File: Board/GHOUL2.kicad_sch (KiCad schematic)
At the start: 32 parts, among them M1 Motor_Servo, U1 Teensy4.1, U2 DS18S20, U4 TPS62133, U5 MS5607-02BA, U6 SAM-M8Q

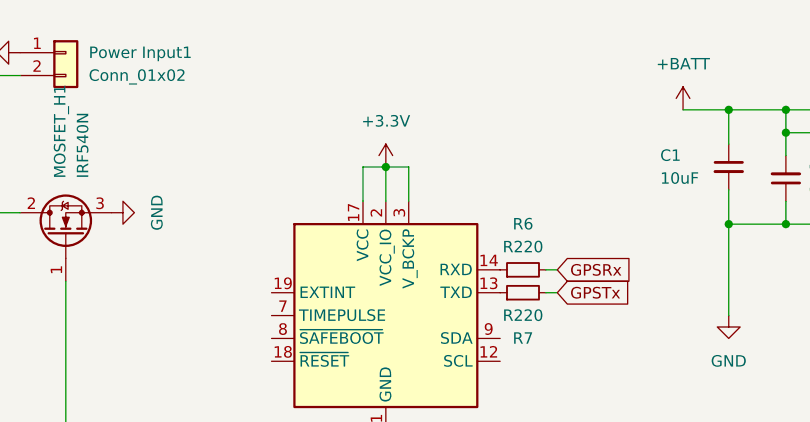
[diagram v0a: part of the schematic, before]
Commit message: decoupling and gps batt
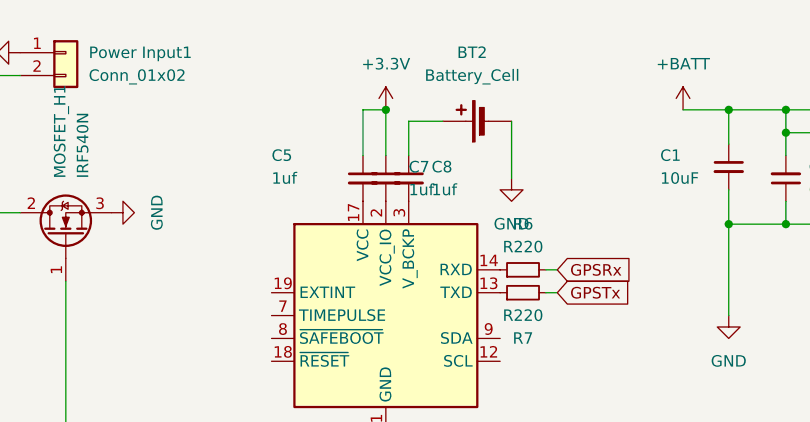
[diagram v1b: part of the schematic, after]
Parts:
- added BT2: Battery_Cell, Battery:BatteryHolder_Keystone_2998_1x6.8mm, symbol Device:Battery_Cell
- added C5, C7, C8: 1uf, Capacitor_SMD:C_0201_0603Metric_Pad0.64x0.40mm_HandSolder, symbol Device:C_Small
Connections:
- net +3.3V: now also C5.1, C7.1; no longer U6.17 (VCC), U6.2 (VCC_IO), U6.3 (V_BCKP)
- net GND: now also BT2.2 (-)
- new net: C5.2, U6.17 (VCC)
- new net: BT2.1 (+), C8.1
- new net: C7.2, U6.2 (VCC_IO)
- new net: C8.2, U6.3 (V_BCKP)
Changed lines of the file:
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@@
   (junction (at 240.03 54.61) (diameter 0) (color 0 0 0 0)
   )
-  (junction (at 166.37 31.75) (diameter 0) (color 0 0 0 0)
-  )
   (junction (at 256.54 43.18) (diameter 0) (color 0 0 0 0)
   )
@@
   (junction (at 30.48 148.59) (diameter 0) (color 0 0 0 0)
   )
+  (junction (at 166.37 25.4) (diameter 0) (color 0 0 0 0)
+  )
   (junction (at 107.95 143.51) (diameter 0) (color 0 0 0 0)
   )
@@
     (stroke (width 0) (type default))
   )
+  (wire (pts (xy 172.72 26.67) (xy 168.91 26.67))
+    (stroke (width 0) (type default))
+  )
   (wire (pts (xy 240.03 54.61) (xy 237.49 54.61))
     (stroke (width 0) (type default))
@@
     (stroke (width 0) (type default))
   )
+  (wire (pts (xy 180.34 26.67) (xy 180.34 33.02))
+    (stroke (width 0) (type default))
+  )
   (wire (pts (xy 30.48 148.59) (xy 53.34 148.59))
     (stroke (width 0) (type default))
@@
     (stroke (width 0) (type default))
   )
+  (wire (pts (xy 163.83 30.48) (xy 163.83 25.4))
+    (stroke (width 0) (type default))
+  )
   (wire (pts (xy 237.49 53.34) (xy 237.49 54.61))
     (stroke (width 0) (type default))
@@
     (stroke (width 0) (type default))
   )
-  (wire (pts (xy 163.83 35.56) (xy 163.83 31.75))
-    (stroke (width 0) (type default))
-  )
   (wire (pts (xy 26.67 168.91) (xy 29.21 168.91))
     (stroke (width 0) (type default))
@@
     (stroke (width 0) (type default))
   )
-  (wire (pts (xy 166.37 31.75) (xy 168.91 31.75))
-    (stroke (width 0) (type default))
-  )
   (wire (pts (xy 26.67 148.59) (xy 26.67 156.21))
     (stroke (width 0) (type default))
@@
     (stroke (width 0) (type default))
   )
-  (wire (pts (xy 168.91 31.75) (xy 168.91 35.56))
-    (stroke (width 0) (type default))
-  )
   (wire (pts (xy 218.44 142.24) (xy 219.71 142.24))
     (stroke (width 0) (type default))
@@
     (stroke (width 0) (type default))
   )
-  (wire (pts (xy 163.83 31.75) (xy 166.37 31.75))
-    (stroke (width 0) (type default))
-  )
   (wire (pts (xy 115.57 21.59) (xy 125.73 21.59))
     (stroke (width 0) (type default))
@@
     (stroke (width 0) (type default))
   )
+  (wire (pts (xy 168.91 26.67) (xy 168.91 30.48))
+    (stroke (width 0) (type default))
+  )
   (wire (pts (xy 222.25 43.18) (xy 227.33 43.18))
     (stroke (width 0) (type default))
@@
     (stroke (width 0) (type default))
   )
-  (wire (pts (xy 166.37 31.75) (xy 166.37 35.56))
+  (wire (pts (xy 166.37 25.4) (xy 166.37 30.48))
     (stroke (width 0) (type default))
   )
@@
   )
   (wire (pts (xy 237.49 54.61) (xy 234.95 54.61))
+    (stroke (width 0) (type default))
+  )
+  (wire (pts (xy 163.83 25.4) (xy 166.37 25.4))
     (stroke (width 0) (type default))
   )
@@
     (property "Intersheetrefs" "${INTERSHEET_REFS}" (at 27.495 41.91 0)
       (effects (font (size 1.27 1.27)) (justify right) hide)
+    )
+  )
+  (symbol (lib_id "Device:C_Small") (at 163.83 33.02 0) (unit 1)
+    (in_bom yes) (on_board yes) (dnp no)
+    (property "Reference" "C5" (at 153.67 30.48 0)
+      (effects (font (size 1.27 1.27)) (justify left))
+    )
+    (property "Value" "1uf" (at 153.67 33.02 0)
+      (effects (font (size 1.27 1.27)) (justify left))
+    )
+    (property "Footprint" "Capacitor_SMD:C_0201_0603Metric_Pad0.64x0.40mm_HandSolder" (at 163.83 33.02 0)
+      (effects (font (size 1.27 1.27)) hide)
+    )
+    (property "Datasheet" "~" (at 163.83 33.02 0)
+      (effects (font (size 1.27 1.27)) hide)
+    )
+    (pin "1")
+    (pin "2")
+    (instances
+      (project "GHOUL2"
+        (path "/a2e390a1-3d20-4e85-b6dd-da84eefdc6ca"
+          (reference "C5") (unit 1)
+        )
+      )
     )
   )
@@
         (path "/a2e390a1-3d20-4e85-b6dd-da84eefdc6ca"
           (reference "#PWR07") (unit 1)
+        )
+      )
+    )
+  )
+  (symbol (lib_id "Device:Battery_Cell") (at 177.8 26.67 90) (unit 1)
+    (in_bom yes) (on_board yes) (dnp no) (fields_autoplaced)
+    (property "Reference" "BT2" (at 175.9585 19.05 90)
+      (effects (font (size 1.27 1.27)))
+    )
+    (property "Value" "Battery_Cell" (at 175.9585 21.59 90)
+      (effects (font (size 1.27 1.27)))
+    )
+    (property "Footprint" "Battery:BatteryHolder_Keystone_2998_1x6.8mm" (at 176.276 26.67 90)
+      (effects (font (size 1.27 1.27)) hide)
+    )
+    (property "Datasheet" "~" (at 176.276 26.67 90)
+      (effects (font (size 1.27 1.27)) hide)
+    )
+    (pin "1")
+    (pin "2")
+    (instances
+      (project "GHOUL2"
+        (path "/a2e390a1-3d20-4e85-b6dd-da84eefdc6ca"
+          (reference "BT2") (unit 1)
         )
       )
@@
     )
   )
+  (symbol (lib_id "Device:C_Small") (at 166.37 33.02 0) (unit 1)
+    (in_bom yes) (on_board yes) (dnp no) (fields_autoplaced)
+    (property "Reference" "C7" (at 168.91 31.7563 0)
+      (effects (font (size 1.27 1.27)) (justify left))
+    )
+    (property "Value" "1uf" (at 168.91 34.2963 0)
+      (effects (font (size 1.27 1.27)) (justify left))
+    )
+    (property "Footprint" "Capacitor_SMD:C_0201_0603Metric_Pad0.64x0.40mm_HandSolder" (at 166.37 33.02 0)
+      (effects (font (size 1.27 1.27)) hide)
+    )
+    (property "Datasheet" "~" (at 166.37 33.02 0)
+      (effects (font (size 1.27 1.27)) hide)
+    )
+    (pin "1")
+    (pin "2")
+    (instances
+      (project "GHOUL2"
+        (path "/a2e390a1-3d20-4e85-b6dd-da84eefdc6ca"
+          (reference "C7") (unit 1)
+        )
+      )
+    )
+  )
   (symbol (lib_id "power:GND") (at 143.51 120.65 270) (unit 1)
     (in_bom yes) (on_board yes) (dnp no)
@@
     )
   )
+  (symbol (lib_name "GND_8") (lib_id "power:GND") (at 180.34 33.02 0) (unit 1)
+    (in_bom yes) (on_board yes) (dnp no) (fields_autoplaced)
+    (property "Reference" "#PWR023" (at 180.34 39.37 0)
+      (effects (font (size 1.27 1.27)) hide)
+    )
+    (property "Value" "GND" (at 180.34 38.1 0)
+      (effects (font (size 1.27 1.27)))
+    )
+    (property "Footprint" "" (at 180.34 33.02 0)
+      (effects (font (size 1.27 1.27)) hide)
+    )
+    (property "Datasheet" "" (at 180.34 33.02 0)
+      (effects (font (size 1.27 1.27)) hide)
+    )
+    (pin "1")
+    (instances
+      (project "GHOUL2"
+        (path "/a2e390a1-3d20-4e85-b6dd-da84eefdc6ca"
+          (reference "#PWR023") (unit 1)
+        )
+      )
+    )
+  )
   (symbol (lib_id "power:GND") (at 156.21 88.9 90) (unit 1)
     (in_bom yes) (on_board yes) (dnp no)
@@
     )
   )
-  (symbol (lib_id "power:+3.3V") (at 166.37 31.75 0) (unit 1)
-    (in_bom yes) (on_board yes) (dnp no) (fields_autoplaced)
-    (property "Reference" "#PWR014" (at 166.37 35.56 0)
-      (effects (font (size 1.27 1.27)) hide)
-    )
-    (property "Value" "+3.3V" (at 166.37 26.67 0)
-      (effects (font (size 1.27 1.27)))
-    )
-    (property "Footprint" "" (at 166.37 31.75 0)
-      (effects (font (size 1.27 1.27)) hide)
-    )
-    (property "Datasheet" "" (at 166.37 31.75 0)
+  (symbol (lib_id "power:+3.3V") (at 166.37 25.4 0) (unit 1)
+    (in_bom yes) (on_board yes) (dnp no) (fields_autoplaced)
+    (property "Reference" "#PWR014" (at 166.37 29.21 0)
+      (effects (font (size 1.27 1.27)) hide)
+    )
+    (property "Value" "+3.3V" (at 166.37 20.32 0)
+      (effects (font (size 1.27 1.27)))
+    )
+    (property "Footprint" "" (at 166.37 25.4 0)
+      (effects (font (size 1.27 1.27)) hide)
+    )
+    (property "Datasheet" "" (at 166.37 25.4 0)
       (effects (font (size 1.27 1.27)) hide)
     )
@@
         )
       )
+    )
+  )
+  (symbol (lib_id "Device:C_Small") (at 168.91 33.02 0) (unit 1)
+    (in_bom yes) (on_board yes) (dnp no) (fields_autoplaced)
+    (property "Reference" "C8" (at 171.45 31.7563 0)
+      (effects (font (size 1.27 1.27)) (justify left))
+    )
+    (property "Value" "1uf" (at 171.45 34.2963 0)
+      (effects (font (size 1.27 1.27)) (justify left))
+    )
+    (property "Footprint" "Capacitor_SMD:C_0201_0603Metric_Pad0.64x0.40mm_HandSolder" (at 168.91 33.02 0)
+      (effects (font (size 1.27 1.27)) hide)
+    )
+    (property "Datasheet" "~" (at 168.91 33.02 0)
+      (effects (font (size 1.27 1.27)) hide)
+    )
+    (pin "1")
+    (pin "2")
+    (instances
+      (project "GHOUL2"
+        (path "/a2e390a1-3d20-4e85-b6dd-da84eefdc6ca"
+          (reference "C8") (unit 1)
+        )
+      )

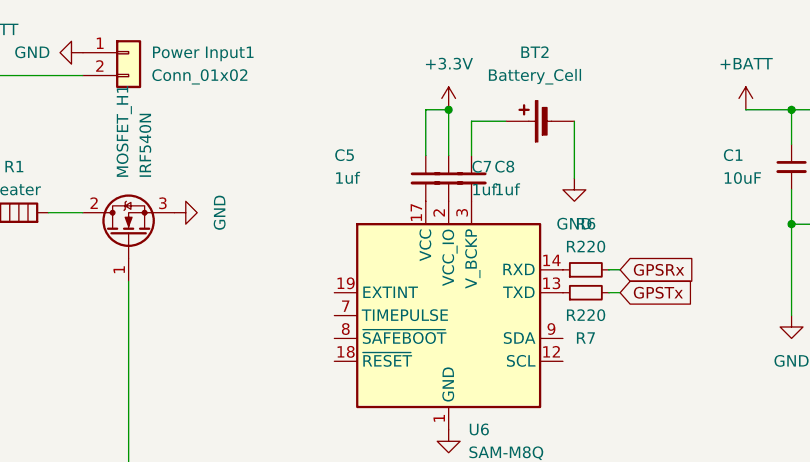
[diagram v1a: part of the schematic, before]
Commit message: fixed caps and things
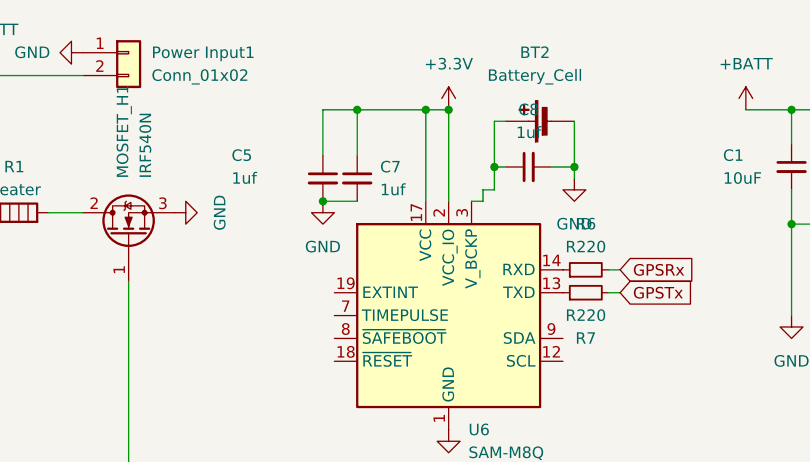
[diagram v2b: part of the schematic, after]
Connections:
- net +3.3V: now also U6.17 (VCC), U6.2 (VCC_IO)
- net GND: now also C5.2, C7.2, C8.2
- net at BT2.1 (+), C8.1: now also U6.3 (V_BCKP)
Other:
- moved on the sheet: C5, C7, C8
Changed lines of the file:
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@@
   (junction (at 29.21 168.91) (diameter 0) (color 0 0 0 0)
   )
+  (junction (at 163.83 25.4) (diameter 0) (color 0 0 0 0)
+  )
   (junction (at 218.44 142.24) (diameter 0) (color 0 0 0 0)
   )
   (junction (at 240.03 54.61) (diameter 0) (color 0 0 0 0)
   )
+  (junction (at 180.34 31.75) (diameter 0) (color 0 0 0 0)
+  )
   (junction (at 256.54 43.18) (diameter 0) (color 0 0 0 0)
   )
+  (junction (at 171.45 31.75) (diameter 0) (color 0 0 0 0)
+  )
+  (junction (at 152.4 35.56) (diameter 0) (color 0 0 0 0)
+  )
   (junction (at 72.39 171.45) (diameter 0) (color 0 0 0 0)
   )
@@
   (junction (at 210.82 38.1) (diameter 0) (color 0 0 0 0)
   )
+  (junction (at 156.21 25.4) (diameter 0) (color 0 0 0 0)
+  )
   (junction (at 237.49 54.61) (diameter 0) (color 0 0 0 0)
   )
@@
     (stroke (width 0) (type default))
   )
+  (wire (pts (xy 170.18 35.56) (xy 168.91 35.56))
+    (stroke (width 0) (type default))
+  )
   (wire (pts (xy 210.82 27.94) (xy 210.82 30.48))
     (stroke (width 0) (type default))
@@
     (stroke (width 0) (type default))
   )
+  (wire (pts (xy 163.83 25.4) (xy 163.83 35.56))
+    (stroke (width 0) (type default))
+  )
+  (wire (pts (xy 172.72 31.75) (xy 171.45 31.75))
+    (stroke (width 0) (type default))
+  )
   (wire (pts (xy 222.25 40.64) (xy 222.25 43.18))
     (stroke (width 0) (type default))
@@
     (stroke (width 0) (type default))
   )
+  (wire (pts (xy 156.21 25.4) (xy 163.83 25.4))
+    (stroke (width 0) (type default))
+  )
   (wire (pts (xy 72.39 171.45) (xy 38.1 171.45))
     (stroke (width 0) (type default))
@@
     (stroke (width 0) (type default))
   )
+  (wire (pts (xy 152.4 35.56) (xy 156.21 35.56))
+    (stroke (width 0) (type default))
+  )
   (wire (pts (xy 237.49 134.62) (xy 233.68 134.62))
     (stroke (width 0) (type default))
@@
     (stroke (width 0) (type default))
   )
-  (wire (pts (xy 172.72 26.67) (xy 168.91 26.67))
+  (wire (pts (xy 171.45 26.67) (xy 172.72 26.67))
     (stroke (width 0) (type default))
   )
@@
     (stroke (width 0) (type default))
   )
-  (wire (pts (xy 180.34 26.67) (xy 180.34 33.02))
+  (wire (pts (xy 180.34 26.67) (xy 180.34 31.75))
+    (stroke (width 0) (type default))
+  )
+  (wire (pts (xy 177.8 31.75) (xy 180.34 31.75))
     (stroke (width 0) (type default))
   )
@@
     (stroke (width 0) (type default))
   )
+  (wire (pts (xy 170.18 34.29) (xy 170.18 35.56))
+    (stroke (width 0) (type default))
+  )
   (wire (pts (xy 256.54 36.83) (xy 256.54 35.56))
     (stroke (width 0) (type default))
@@
     (stroke (width 0) (type default))
   )
+  (wire (pts (xy 180.34 31.75) (xy 180.34 33.02))
+    (stroke (width 0) (type default))
+  )
   (wire (pts (xy 184.15 45.72) (xy 185.42 45.72))
     (stroke (width 0) (type default))
@@
     (stroke (width 0) (type default))
   )
-  (wire (pts (xy 163.83 30.48) (xy 163.83 25.4))
+  (wire (pts (xy 152.4 30.48) (xy 152.4 25.4))
     (stroke (width 0) (type default))
   )
@@
     (stroke (width 0) (type default))
   )
+  (wire (pts (xy 171.45 31.75) (xy 171.45 34.29))
+    (stroke (width 0) (type default))
+  )
   (wire (pts (xy 219.71 134.62) (xy 227.33 134.62))
     (stroke (width 0) (type default))
@@
     (stroke (width 0) (type default))
   )
+  (wire (pts (xy 166.37 25.4) (xy 166.37 35.56))
+    (stroke (width 0) (type default))
+  )
   (wire (pts (xy 26.67 148.59) (xy 26.67 156.21))
     (stroke (width 0) (type default))
@@
     (stroke (width 0) (type default))
   )
+  (wire (pts (xy 163.83 25.4) (xy 166.37 25.4))
+    (stroke (width 0) (type default))
+  )
   (wire (pts (xy 130.81 44.45) (xy 130.81 64.77))
     (stroke (width 0) (type default))
@@
     (stroke (width 0) (type default))
   )
+  (wire (pts (xy 171.45 34.29) (xy 170.18 34.29))
+    (stroke (width 0) (type default))
+  )
   (wire (pts (xy 130.81 64.77) (xy 96.52 64.77))
     (stroke (width 0) (type default))
@@
     (stroke (width 0) (type default))
   )
-  (wire (pts (xy 168.91 26.67) (xy 168.91 30.48))
+  (wire (pts (xy 171.45 26.67) (xy 171.45 31.75))
     (stroke (width 0) (type default))
   )
@@
     (stroke (width 0) (type default))
   )
-  (wire (pts (xy 166.37 25.4) (xy 166.37 30.48))
+  (wire (pts (xy 156.21 25.4) (xy 156.21 30.48))
     (stroke (width 0) (type default))
   )
@@
     (stroke (width 0) (type default))
   )
-  (wire (pts (xy 163.83 25.4) (xy 166.37 25.4))
+  (wire (pts (xy 152.4 25.4) (xy 156.21 25.4))
     (stroke (width 0) (type default))
   )
@@
     )
   )
-  (symbol (lib_id "Device:C_Small") (at 163.83 33.02 0) (unit 1)
+  (symbol (lib_id "Device:C_Small") (at 152.4 33.02 0) (unit 1)
     (in_bom yes) (on_board yes) (dnp no)
-    (property "Reference" "C5" (at 153.67 30.48 0)
-      (effects (font (size 1.27 1.27)) (justify left))
-    )
-    (property "Value" "1uf" (at 153.67 33.02 0)
-      (effects (font (size 1.27 1.27)) (justify left))
-    )
-    (property "Footprint" "Capacitor_SMD:C_0201_0603Metric_Pad0.64x0.40mm_HandSolder" (at 163.83 33.02 0)
-      (effects (font (size 1.27 1.27)) hide)
-    )
-    (property "Datasheet" "~" (at 163.83 33.02 0)
+    (property "Reference" "C5" (at 142.24 30.48 0)
+      (effects (font (size 1.27 1.27)) (justify left))
+    )
+    (property "Value" "1uf" (at 142.24 33.02 0)
+      (effects (font (size 1.27 1.27)) (justify left))
+    )
+    (property "Footprint" "Capacitor_SMD:C_0201_0603Metric_Pad0.64x0.40mm_HandSolder" (at 152.4 33.02 0)
+      (effects (font (size 1.27 1.27)) hide)
+    )
+    (property "Datasheet" "~" (at 152.4 33.02 0)
       (effects (font (size 1.27 1.27)) hide)
     )
@@
         (path "/a2e390a1-3d20-4e85-b6dd-da84eefdc6ca"
           (reference "U2") (unit 1)
+        )
+      )
+    )
+  )
+  (symbol (lib_name "GND_9") (lib_id "power:GND") (at 152.4 35.56 0) (unit 1)
+    (in_bom yes) (on_board yes) (dnp no) (fields_autoplaced)
+    (property "Reference" "#PWR024" (at 152.4 41.91 0)
+      (effects (font (size 1.27 1.27)) hide)
+    )
+    (property "Value" "GND" (at 152.4 40.64 0)
+      (effects (font (size 1.27 1.27)))
+    )
+    (property "Footprint" "" (at 152.4 35.56 0)
+      (effects (font (size 1.27 1.27)) hide)
+    )
+    (property "Datasheet" "" (at 152.4 35.56 0)
+      (effects (font (size 1.27 1.27)) hide)
+    )
+    (pin "1")
+    (instances
+      (project "GHOUL2"
+        (path "/a2e390a1-3d20-4e85-b6dd-da84eefdc6ca"
+          (reference "#PWR024") (unit 1)
         )
       )
@@
     )
   )
-  (symbol (lib_id "Device:C_Small") (at 166.37 33.02 0) (unit 1)
-    (in_bom yes) (on_board yes) (dnp no) (fields_autoplaced)
-    (property "Reference" "C7" (at 168.91 31.7563 0)
-      (effects (font (size 1.27 1.27)) (justify left))
-    )
-    (property "Value" "1uf" (at 168.91 34.2963 0)
-      (effects (font (size 1.27 1.27)) (justify left))
-    )
-    (property "Footprint" "Capacitor_SMD:C_0201_0603Metric_Pad0.64x0.40mm_HandSolder" (at 166.37 33.02 0)
-      (effects (font (size 1.27 1.27)) hide)
-    )
-    (property "Datasheet" "~" (at 166.37 33.02 0)
+  (symbol (lib_id "Device:C_Small") (at 156.21 33.02 0) (unit 1)
+    (in_bom yes) (on_board yes) (dnp no) (fields_autoplaced)
+    (property "Reference" "C7" (at 158.75 31.7563 0)
+      (effects (font (size 1.27 1.27)) (justify left))
+    )
+    (property "Value" "1uf" (at 158.75 34.2963 0)
+      (effects (font (size 1.27 1.27)) (justify left))
+    )
+    (property "Footprint" "Capacitor_SMD:C_0201_0603Metric_Pad0.64x0.40mm_HandSolder" (at 156.21 33.02 0)
+      (effects (font (size 1.27 1.27)) hide)
+    )
+    (property "Datasheet" "~" (at 156.21 33.02 0)
       (effects (font (size 1.27 1.27)) hide)
     )
@@
     )
   )
-  (symbol (lib_id "Device:C_Small") (at 168.91 33.02 0) (unit 1)
-    (in_bom yes) (on_board yes) (dnp no) (fields_autoplaced)
-    (property "Reference" "C8" (at 171.45 31.7563 0)
-      (effects (font (size 1.27 1.27)) (justify left))
-    )
-    (property "Value" "1uf" (at 171.45 34.2963 0)
-      (effects (font (size 1.27 1.27)) (justify left))
-    )
-    (property "Footprint" "Capacitor_SMD:C_0201_0603Metric_Pad0.64x0.40mm_HandSolder" (at 168.91 33.02 0)
-      (effects (font (size 1.27 1.27)) hide)
-    )
-    (property "Datasheet" "~" (at 168.91 33.02 0)
-      (effects (font (size 1.27 1.27)) hide)
-    )
+  (symbol (lib_id "Device:C_Small") (at 175.26 31.75 90) (unit 1)
+    (in_bom yes) (on_board yes) (dnp no) (fields_autoplaced)
+    (property "Reference" "C8" (at 175.2663 25.4 90)
+      (effects (font (size 1.27 1.27)))
+    )
+    (property "Value" "1uf" (at 175.2663 27.94 90)
+      (effects (font (size 1.27 1.27)))
+    )
+    (property "Footprint" "Capacitor_SMD:C_0201_0603Metric_Pad0.64x0.40mm_HandSolder" (at 175.26 31.75 0)
+      (effects (font (size 1.27 1.27)) hide)
+    )
+    (property "Datasheet" "~" (at 175.26 31.75 0)
+      (effects (font (size 1.27 1.27)) hide)
+    )
